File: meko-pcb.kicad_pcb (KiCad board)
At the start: 4 copper layers, 37 x 69 mm, 158 parts, among them IC1 AS5600-ASOM, IC2 TCAL9538RSVR, IC3 LP5912-3.3DRVR, IC4 ES9218PQ, IC5 BQ27427YZFR, J1 GDEY0154D67, J2 MEM2090-00-145-00-A, J3 USB_C_Receptacle_USB2.0_16P, J4 SJ2-35954B-SMT-TR, M1 HD-EMB1204-SM, Q1 SS8050, Q2 SS8050, Q3 SS8050, Q4 Si1308EDL, SW1 SW_Push, SW2 SW_Push, SW3 SW_Push, SW4 SW_Push, SW5 SW_Push, SW6 SW_Push, SW7 SW_Push, U1 ESP32-PICO-MINI-02, U10 LP5907SNX-1.8/NOPB, U2 BQ24075RGT, U3 LP5907SNX-3.3/NOPB, U4 LP5907SNX-3.3/NOPB, U6 LP5907SNX-3.3/NOPB, U7 LP5907SNX-1.8/NOPB, U8 USBLC6-2SC6, U9 CP2102N-Axx-xQFN24, Y1 ECS-2520SMV-500-GP-TR

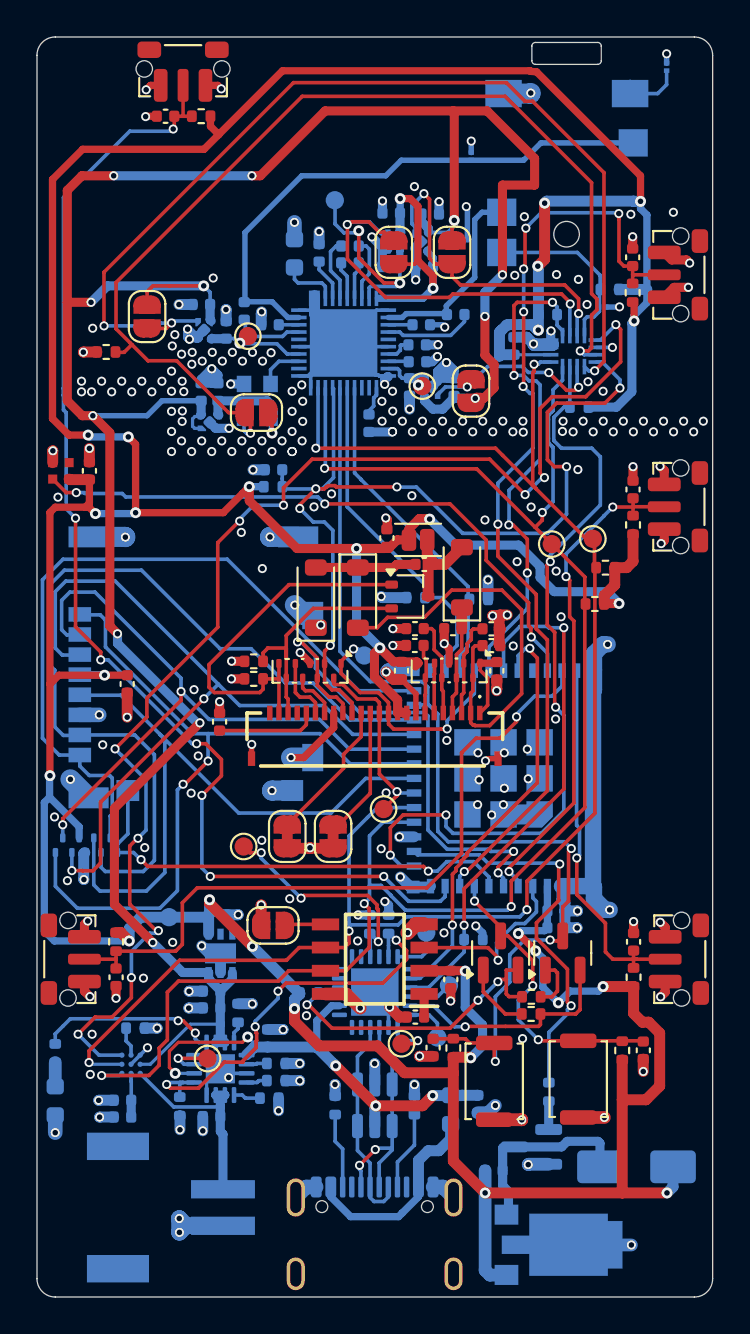
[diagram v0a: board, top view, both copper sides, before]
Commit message: minor stuff
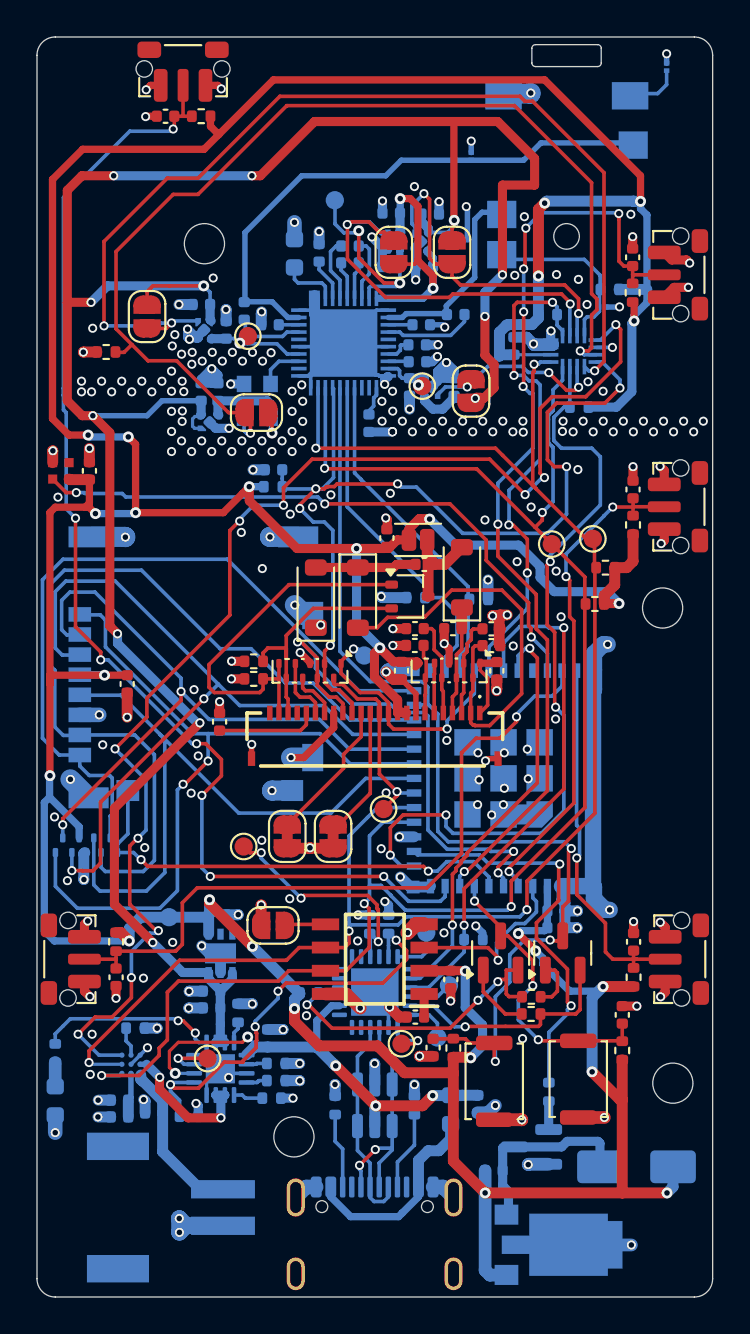
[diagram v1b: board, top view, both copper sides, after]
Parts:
- added H1: MountingHole, MountingHole:MountingHole_2.2mm_M2, F.Cu at (82.7, 32.8)
- added H2: MountingHole, MountingHole:MountingHole_2.2mm_M2, F.Cu at (107.8, 52.8)
- added H3: MountingHole, MountingHole:MountingHole_2.2mm_M2, F.Cu at (87.6, 81.7)
- added H4: MountingHole, MountingHole:MountingHole_2.2mm_M2, F.Cu at (108.3, 78.8)
- moved C24 3.17 mm to (79.9, 80.4)
- moved C6 2.26 mm to (105.5, 75.0), turned to 90 degrees
- moved R18 0.74 mm to (81.8, 80.6), turned to 0 degrees
- moved C57 0.16 mm to (78.0, 79.7)
- moved C58 0.16 mm to (78.0, 80.6)
- moved R16 0.13 mm to (86.3, 79.6)
- moved J4 0.12 mm to (102.5, 27.9)
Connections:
- IC5 pad C2: REG-OUT -> /power/SRX
- U2 pad 2: +BATT -> /power/SRX
- U2 pad 3: +BATT -> /power/SRX
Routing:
- net /power/SRX: track 0.00 -> 8.27 mm, vias 0 -> 2
- net REG-OUT: track 144.1 -> 137.8 mm
- net +3V3: track 284.3 -> 280.9 mm, vias 28 -> 27
- net +BATT: track 11.3 -> 9.29 mm
- net Net-(D9-A2): track 3.64 -> 3.02 mm
- net /AUDIO_MLCK_EN: track 58.1 -> 58.7 mm
- net /PWR_EN_USB: track 23.0 -> 23.5 mm
- net GND: track 191.6 -> 191.5 mm, vias 260 -> 259
